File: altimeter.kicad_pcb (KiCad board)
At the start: 2 copper layers, 38.1 x 22.9 mm, 25 parts, among them J1 Conn_01x03_Male, J2 Conn_01x05_Male, J3 Conn_01x05_Male, J4 Conn_01x03_Male, Q1 Q_NMOS_DGS, U1 TLV760, U2 test, U3 accel, U4 RN4871, U5 EEPROM, U6 BMP280

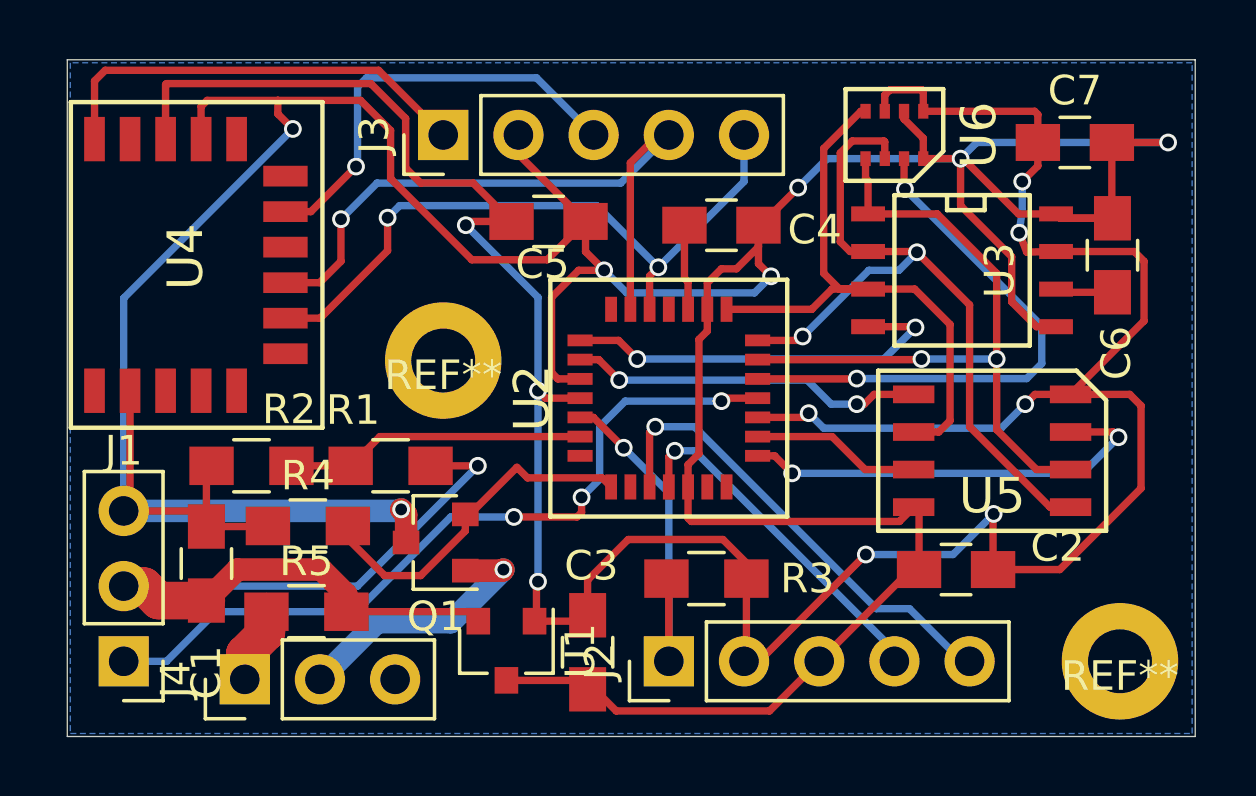
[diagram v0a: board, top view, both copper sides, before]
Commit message: Dev3
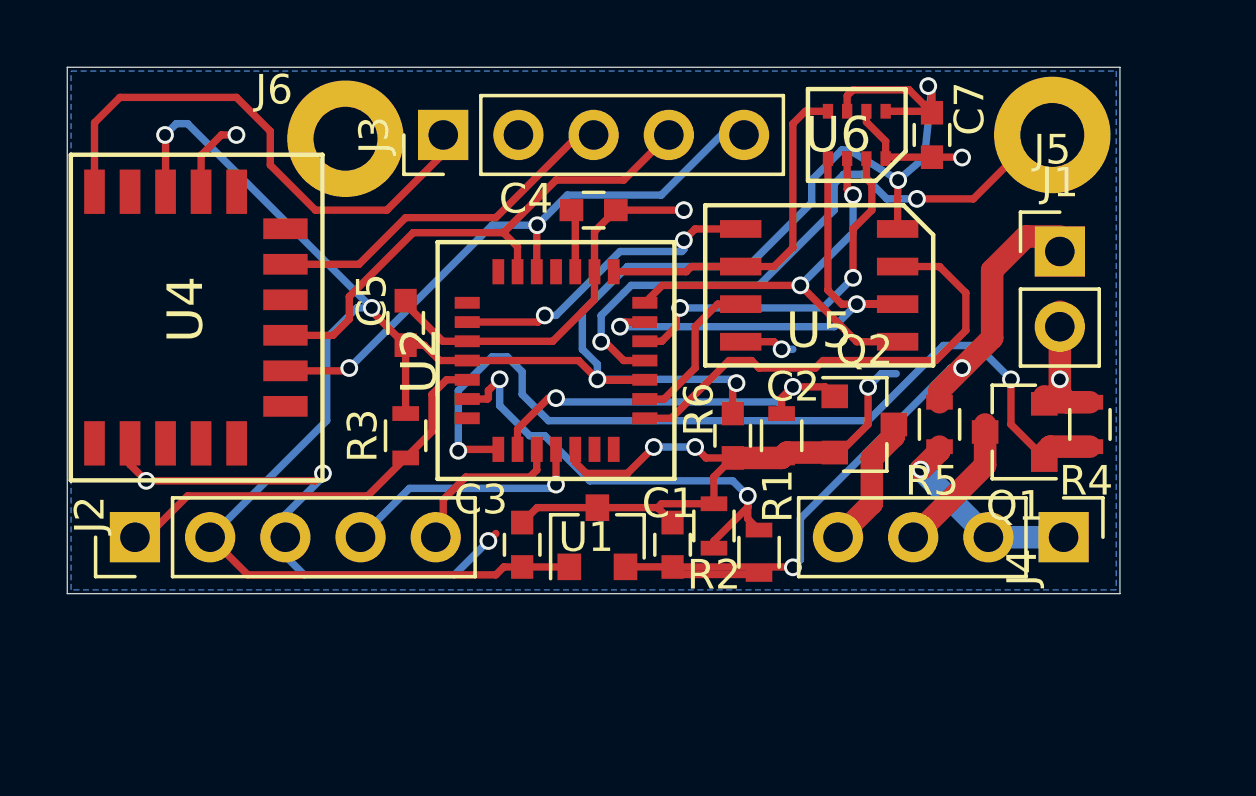
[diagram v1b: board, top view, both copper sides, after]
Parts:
- removed C6: 1u, Capacitors_SMD:C_0805_HandSoldering
- removed REF** (x2): MountingHole_2.5mm_Pad_Via, lib:2-56_hole
- removed U3: accel, SMD_Packages:SOIC-8-N
- added J5: Conn_01x01_Male, lib:2-56_hole, F.Cu at (96.8, 50.8)
- added J6: Conn_01x01_Male, lib:2-56_hole, F.Cu at (72.9, 50.9)
- added Q2: Q_NMOS_DGS, TO_SOT_Packages_SMD:SOT-23, F.Cu at (90.4, 60.6)
- added R6: 100k, Resistors_SMD:R_0603, F.Cu at (87.6, 61.0)
- C1, C2, C3, C4, C5, C7: footprint Capacitors_SMD:C_0805_HandSoldering -> Capacitors_SMD:C_0603
- J1: footprint Pin_Headers:Pin_Header_Straight_1x03_Pitch2.54mm -> Pin_Headers:Pin_Header_Straight_1x02_Pitch2.54mm
- J4: footprint Pin_Headers:Pin_Header_Straight_1x03_Pitch2.54mm -> Pin_Headers:Pin_Header_Straight_1x04_Pitch2.54mm
- R1, R2, R3, R4: footprint Resistors_SMD:R_0805_HandSoldering -> Resistors_SMD:R_0603
- R5: value 100k -> 5; footprint Resistors_SMD:R_0805_HandSoldering -> Resistors_SMD:R_0603
- moved J1 34.5 mm to (97.0, 54.7), turned to 0 degrees
- moved J4 28.1 mm to (97.2, 64.4), turned to 270 degrees
- moved R4 26.6 mm to (98.0, 60.6), turned to 270 degrees
- moved R5 22.3 mm to (93.0, 60.6), turned to 90 degrees
- moved Q1 19.9 mm to (95.5, 60.8)
- moved J2 18.5 mm to (65.8, 64.4)
- moved C1 15.8 mm to (83.9, 64.6)
- moved R2 15.8 mm to (85.3, 64.0), turned to 270 degrees
- moved R1 12.8 mm to (86.9, 64.9), turned to 270 degrees
- moved R3 11.2 mm to (74.9, 61.0), turned to 90 degrees
- moved C2 8.79 mm to (86.0, 61.0), turned to 270 degrees
- moved U5 8.08 mm to (88.9, 55.9)
- moved C5 5.92 mm to (74.9, 57.1), turned to 90 degrees
- moved U1 4.91 mm to (81.4, 64.4), turned to 90 degrees
- moved C7 4.83 mm to (92.7, 50.8), turned to 270 degrees
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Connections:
- J1 pad 1: DEBUG -> VIN
- J1 pad 2: VIN -> VSS
- J4 pad 2: Net-(J4-Pad2) -> Net-(J4-Pad1)
- J4 pad 3: (no net) -> Net-(J4-Pad3)
- Q1 pad 1: Net-(J4-Pad2) -> Pyro1
- Q1 pad 2: Pyro1 -> VSS
- Q1 pad 3: VSS -> Net-(J4-Pad3)
- U2 pad 2: (no net) -> Pyro2
- U2 pad 22: Net-(U2-Pad22) -> (no net)
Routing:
- net VSS: track 152.5 -> 73.3 mm, vias 7 -> 11
- net +3V3: track 102.9 -> 82.7 mm, vias 9 -> 6
- net Pyro1: track 12.0 -> 30.2 mm, vias 0 -> 2
- net Pyro2: track 0.00 -> 13.8 mm, vias 0 -> 2
- net Net-(U2-Pad22): track 13.6 -> 0.00 mm, vias 2 -> 0
- net SDO: track 25.8 -> 14.7 mm
- net PGC: track 16.0 -> 5.92 mm, vias 1 -> 0
- net Net-(J4-Pad2): track 9.03 -> 0.00 mm, vias 1 -> 0
- net SDI: track 20.8 -> 11.9 mm
- net Net-(U2-Pad12): track 18.7 -> 12.6 mm
- net SCK: track 23.5 -> 17.6 mm
- net Net-(R1-Pad1): track 10.2 -> 15.6 mm, vias 0 -> 2
- net Net-(J4-Pad3): track 0.00 -> 4.82 mm
- net U1RX: track 22.5 -> 17.7 mm, vias 1 -> 0
- net DEBUG: track 26.4 -> 21.8 mm, vias 3 -> 2
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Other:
- board size 38.1 x 22.9 mm -> 35.6 x 17.8 mm
- board text added: "FlightSketch DEV3 vSK01.00 2018-10-04 flightsketch.com"
- board text removed: "Flight Sketch DEV2 vSK01.00 2018-04-28 Russ Parrish"
